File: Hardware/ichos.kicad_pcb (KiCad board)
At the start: 2 copper layers, 1 part, among them J1 629722000214

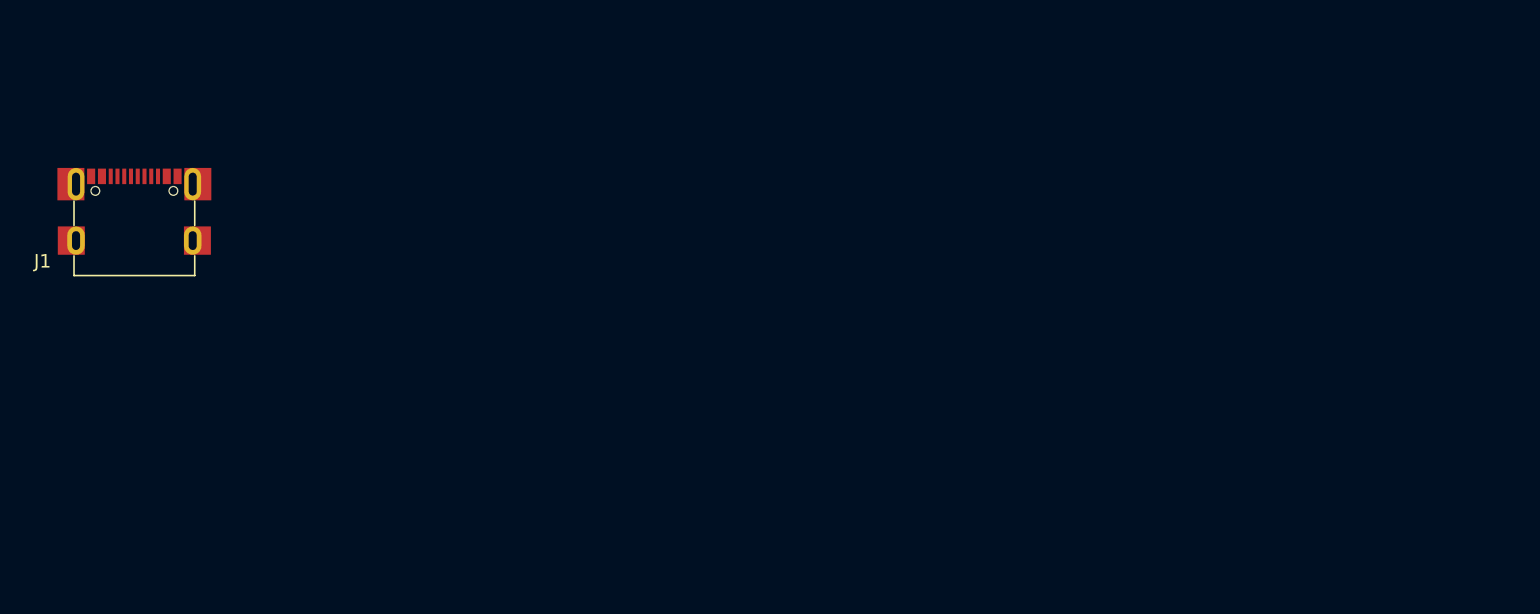
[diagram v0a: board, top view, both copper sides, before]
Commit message: power
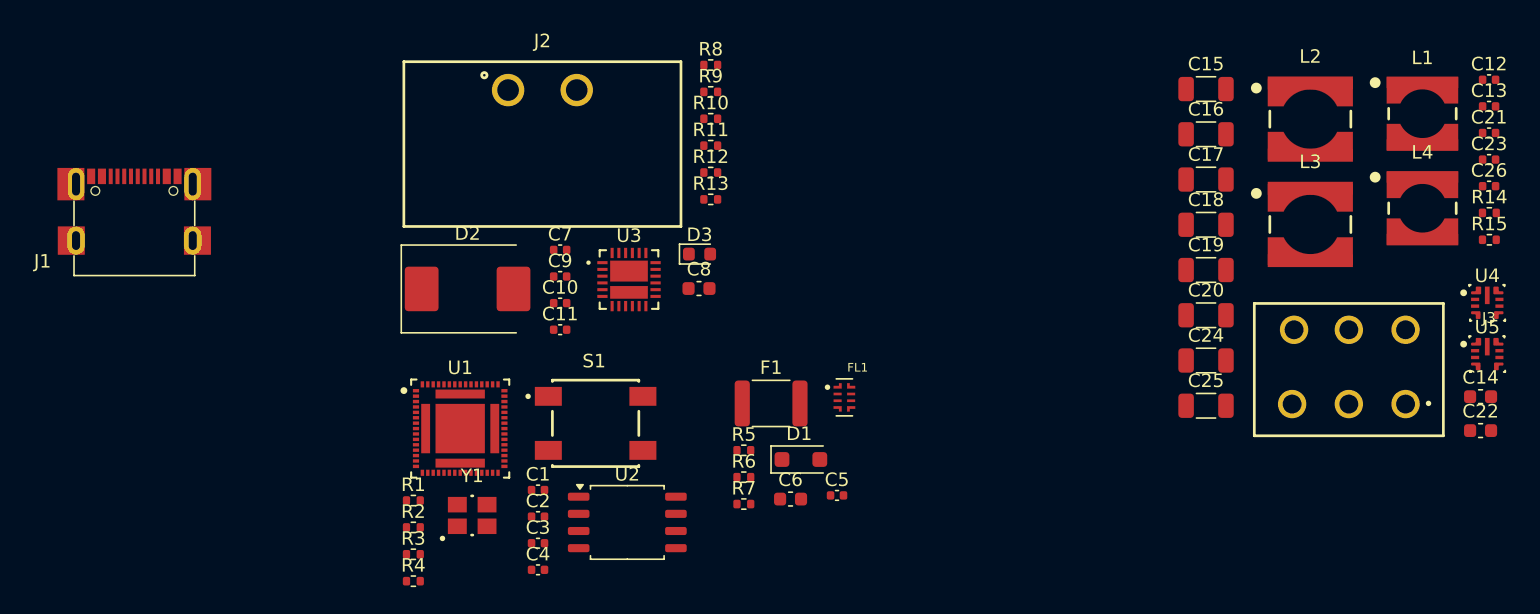
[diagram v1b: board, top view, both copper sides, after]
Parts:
- added C1: 16pF, Capacitor_SMD:C_0402_1005Metric, F.Cu at (87.9, 101.0)
- added C10: 2.2nF, Capacitor_SMD:C_0402_1005Metric, F.Cu at (89.6, 87.2)
- added C11: 4.7nF, Capacitor_SMD:C_0402_1005Metric, F.Cu at (89.6, 89.2)
- added C12: 100nF, Capacitor_SMD:C_0402_1005Metric, F.Cu at (158.4, 70.7)
- added C13: 100nF, Capacitor_SMD:C_0402_1005Metric, F.Cu at (158.4, 72.6)
- added C14: 1uF, Capacitor_SMD:C_0603_1608Metric, F.Cu at (157.7, 94.1)
- added C15: 22uF, Capacitor_SMD:C_1206_3216Metric, F.Cu at (137.4, 71.4)
- added C16: 22uF, Capacitor_SMD:C_1206_3216Metric, F.Cu at (137.4, 74.7)
- added C17: 22uF, Capacitor_SMD:C_1206_3216Metric, F.Cu at (137.4, 78.1)
- added C18: 22uF, Capacitor_SMD:C_1206_3216Metric, F.Cu at (137.4, 81.4)
- added C19: 22uF, Capacitor_SMD:C_1206_3216Metric, F.Cu at (137.4, 84.8)
- added C2: 100nF, Capacitor_SMD:C_0402_1005Metric, F.Cu at (87.9, 103.0)
- added C20: 22uF, Capacitor_SMD:C_1206_3216Metric, F.Cu at (137.4, 88.1)
- added C21: 100nF, Capacitor_SMD:C_0402_1005Metric, F.Cu at (158.4, 74.6)
- added C22: 1uF, Capacitor_SMD:C_0603_1608Metric, F.Cu at (157.7, 96.7)
- added C23: 100nF, Capacitor_SMD:C_0402_1005Metric, F.Cu at (158.4, 76.6)
- added C24: 22uF, Capacitor_SMD:C_1206_3216Metric, F.Cu at (137.4, 91.5)
- added C25: 22uF, Capacitor_SMD:C_1206_3216Metric, F.Cu at (137.4, 94.8)
- added C26: 22pF, Capacitor_SMD:C_0402_1005Metric, F.Cu at (158.4, 78.5)
- added C3: 16pF, Capacitor_SMD:C_0402_1005Metric, F.Cu at (87.9, 105.0)
- added C4: 100nF, Capacitor_SMD:C_0402_1005Metric, F.Cu at (87.9, 107.0)
- added C5: 100nF, Capacitor_SMD:C_0402_1005Metric, F.Cu at (110.1, 101.5)
- added C6: 1uF, Capacitor_SMD:C_0603_1608Metric, F.Cu at (106.6, 101.7)
- added C7: 100nF, Capacitor_SMD:C_0402_1005Metric, F.Cu at (89.6, 83.3)
- added C8: 1uF, Capacitor_SMD:C_0603_1608Metric, F.Cu at (99.8, 86.1)
- added C9: 22pF, Capacitor_SMD:C_0402_1005Metric, F.Cu at (89.6, 85.2)
- added D1: SKM14, Diode_SMD:D_SOD-123F, F.Cu at (107.4, 98.8)
- added D2: 824550121, Diode_SMD:D_SMC, F.Cu at (82.7, 86.2)
- added D3: LED, LED_SMD:LED_0603_1608Metric, F.Cu at (99.9, 83.6)
- added F1: 0ZCG0035FF2C, Fuse:Fuse_1812_4532Metric, F.Cu at (105.2, 94.6)
- added FL1: ECMF02-4CMX8, ichos:ECMF02-4CMX8, F.Cu at (110.6, 94.2)
- added J2: 691317510002, ichos:691317510002, F.Cu at (88.3, 71.4)
- added J3: 64900621122, ichos:64900621122, F.Cu at (148.0, 92.1)
- added L1: 8.2uH, ichos:744042008, F.Cu at (153.4, 73.2)
- added L2: 22uH, ichos:744053220, F.Cu at (145.1, 73.6)
- added L3: 22uH, ichos:744053220, F.Cu at (145.1, 81.4)
- added L4: 8.2uH, ichos:744042008, F.Cu at (153.4, 80.2)
- added R1: 4K7, Resistor_SMD:R_0402_1005Metric, F.Cu at (78.7, 101.8)
- added R10: 1M, Resistor_SMD:R_0402_1005Metric, F.Cu at (100.7, 73.6)
- added R11: 1.5K, Resistor_SMD:R_0402_1005Metric, F.Cu at (100.7, 75.5)
- added R12: 10K, Resistor_SMD:R_0402_1005Metric, F.Cu at (100.7, 77.5)
- added R13: 270R, Resistor_SMD:R_0402_1005Metric, F.Cu at (100.7, 79.5)
- added R14: 33.2K, Resistor_SMD:R_0402_1005Metric, F.Cu at (158.4, 80.5)
- added R15: 43.2K, Resistor_SMD:R_0402_1005Metric, F.Cu at (158.4, 82.5)
- added R2: 1M, Resistor_SMD:R_0402_1005Metric, F.Cu at (78.7, 103.8)
- added R3: 10K, Resistor_SMD:R_0402_1005Metric, F.Cu at (78.7, 105.8)
- added R4: 680R, Resistor_SMD:R_0402_1005Metric, F.Cu at (78.7, 107.8)
- added R5: 10K, Resistor_SMD:R_0402_1005Metric, F.Cu at (103.2, 98.1)
- added R6: 5K1, Resistor_SMD:R_0402_1005Metric, F.Cu at (103.2, 100.1)
- added R7: 5K1, Resistor_SMD:R_0402_1005Metric, F.Cu at (103.2, 102.1)
- added R8: 270R, Resistor_SMD:R_0402_1005Metric, F.Cu at (100.7, 69.6)
- added R9: 180K, Resistor_SMD:R_0402_1005Metric, F.Cu at (100.7, 71.6)
- added S1: 430481031816, ichos:430481031816, F.Cu at (92.2, 96.1)
- added U1: XU316-1024-QF60B-C24, ichos:XU316-1024-QF60B-C32, F.Cu at (82.2, 96.5)
- added U2: W25Q80EWSNIG, Package_SO:SOIC-8_5.23x5.23mm_P1.27mm, F.Cu at (94.5, 103.5)
- added U3: TPS259804ONRGE, ichos:TPS259804ONRGER, F.Cu at (94.7, 85.5)
- added U4: LMR43610MB3RPER, ichos:LMR43610MB3RPER, F.Cu at (158.2, 87.2)
- added U5: LMR43610MB3RPER, ichos:LMR43610MB3RPER, F.Cu at (158.2, 91.0)
- added Y1: 24.0MHz, ichos:830108340709, F.Cu at (83.1, 102.9)
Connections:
- J1 pad A1: (no net) -> GND
- J1 pad A12: (no net) -> GND
- J1 pad A4: (no net) -> Net-(FL1-VBUS)
- J1 pad A5: (no net) -> Net-(J1-CC1)
- J1 pad A6: (no net) -> Net-(FL1-D+-Pad3)
- J1 pad A7: (no net) -> Net-(FL1-D--Pad2)
- J1 pad A8: (no net) -> unconnected-(J1-SBU1-PadA8)
- J1 pad A9: (no net) -> Net-(FL1-VBUS)
- J1 pad B1: (no net) -> GND
- J1 pad B12: (no net) -> GND
- J1 pad B4: (no net) -> Net-(FL1-VBUS)
- J1 pad B5: (no net) -> Net-(J1-CC2)
- J1 pad B6: (no net) -> Net-(FL1-D+-Pad3)
- J1 pad B7: (no net) -> Net-(FL1-D--Pad2)
- J1 pad B8: (no net) -> unconnected-(J1-SBU2-PadB8)
- J1 pad B9: (no net) -> Net-(FL1-VBUS)
- J1 pad S1: (no net) -> Net-(J1-SHIELD)
